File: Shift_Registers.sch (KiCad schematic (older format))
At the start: 3 parts

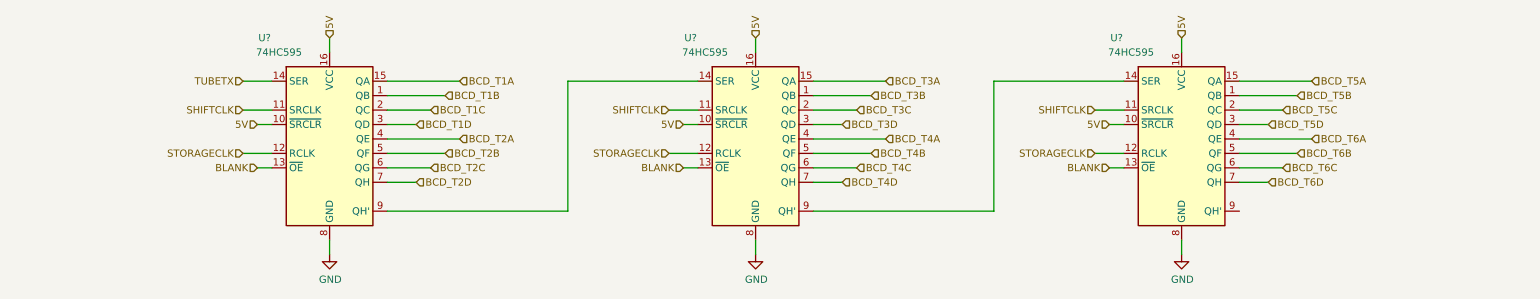
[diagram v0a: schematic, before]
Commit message: Finished draft schema
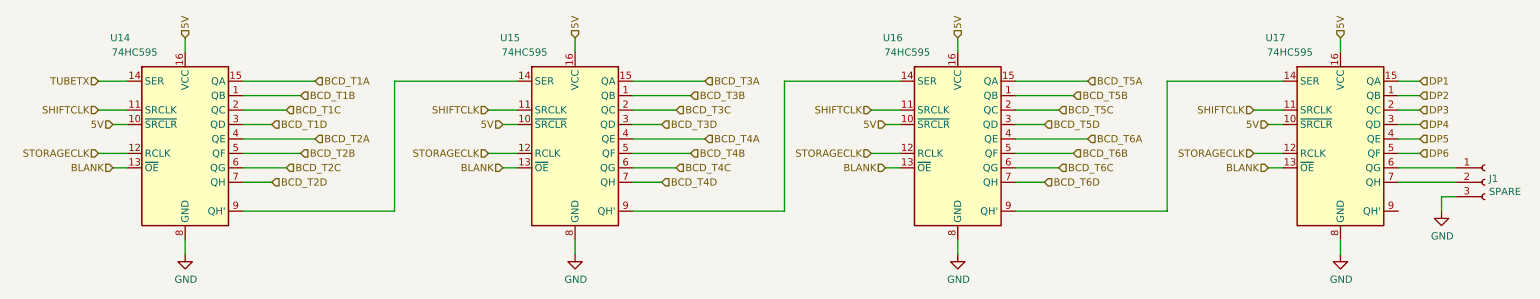
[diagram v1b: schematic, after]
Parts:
- added J1: SPARE, symbol Connector:Conn_01x03_Female
- added U17: 74HC595, symbol 74xx:74HC595
- gave numbers to parts that had none: 3
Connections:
- net 5V: now also U17.10 (~SRCLR), U17.16 (VCC)
- net BLANK: now also U17.13 (~OE)
- net GND: now also J1.3 (Pin_3), U17.8 (GND)
- net SHIFTCLK: now also U17.11 (SRCLK)
- net STORAGECLK: now also U17.12 (RCLK)
- net at U16.9 (QH'): now also U17.14 (SER)
- new net: J1.1 (Pin_1), U17.6 (QG)
- new net: J1.2 (Pin_2), U17.7 (QH)
- new net DP1: U17.15 (QA)
- new net DP2: U17.1 (QB)
- new net DP3: U17.2 (QC)
- new net DP4: U17.3 (QD)
- new net DP5: U17.4 (QE)
- new net DP6: U17.5 (QF)
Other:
- moved on the sheet: U14, U15, U16
